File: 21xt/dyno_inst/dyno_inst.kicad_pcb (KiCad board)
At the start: 4 copper layers, 160 parts, among them IC1 MCP1502T-25E_CHY, IC2 TC7660SEOA713, IC3 MCP1502T-25E_CHY, J1 Conn_01x05, J3 Conn_01x03, J4 Barrel_Jack, J5 Conn_01x06, J6 Conn_01x04, U1 MAX14931FASE+, U10 LT3032IDE-5-TRPBF, U11 NCV8184DR2G, U12 1SS362FV_L3F, U13 1SS362FV_L3F, U14 ADA4807-2ARM, U15 ADA4807-2ARM, U16 ADA4945-1ACPZ-R2, U17 1SS362FV_L3F, U18 1SS362FV_L3F, U19 ADA4807-1, U2 MAX14930FASE+, U20 ADA4807-1, U22 ADA4945-1ACPZ-R2, U23 CPC1017N, U24 LT3032IDE-5-TRPBF, U3 AD7175-2BRUZ, U4 DEV-16771, U5 LT3032IDE-5-TRPBF, U6 1S4E_1.5U, U7 R-78E5.0-0.5, U8 TL431DBZ, U9 TL431DBZ

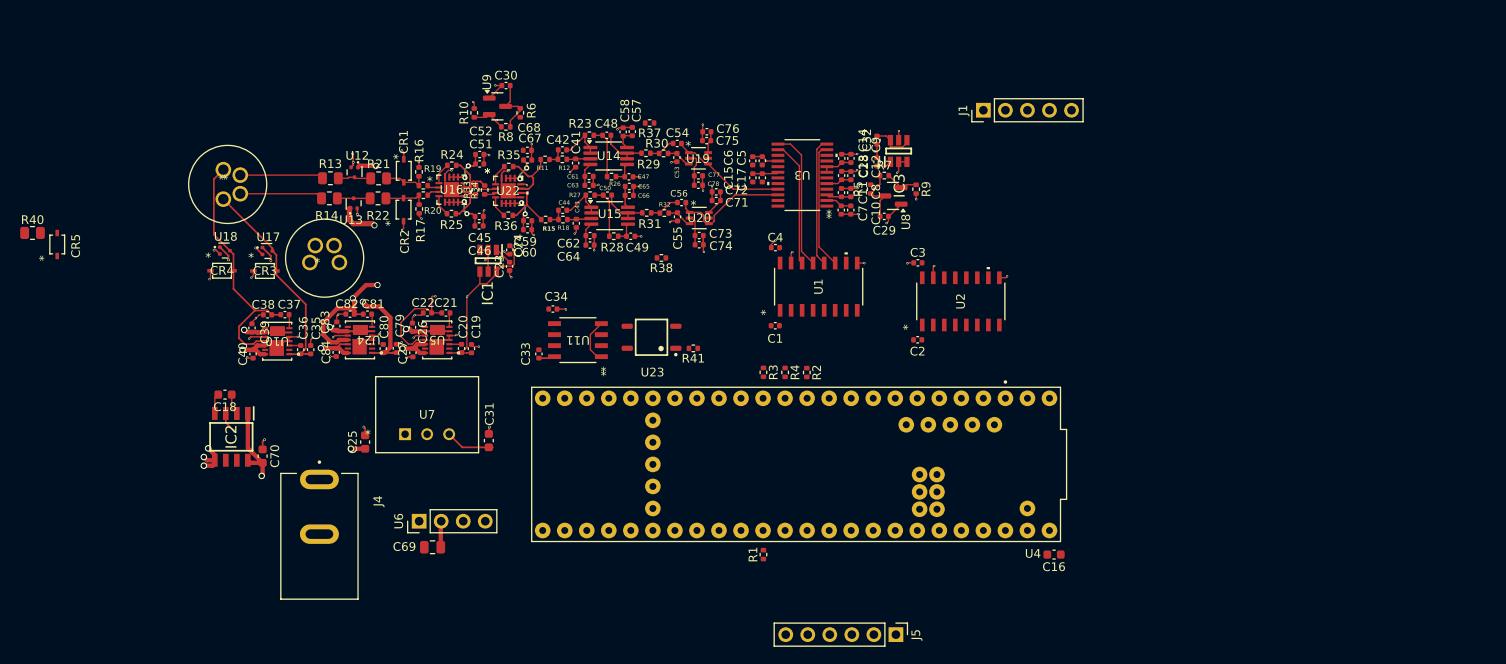
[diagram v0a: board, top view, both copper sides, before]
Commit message: scuffedd
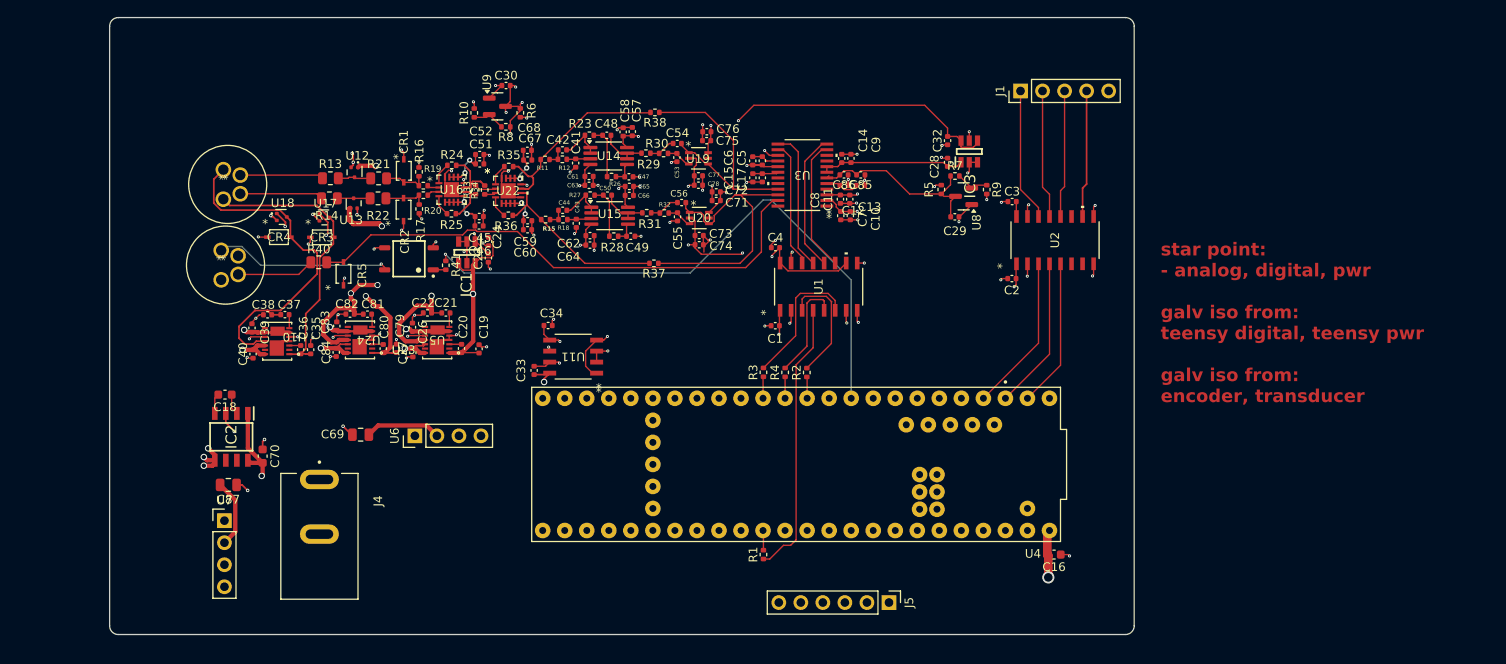
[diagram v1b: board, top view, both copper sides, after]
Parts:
- removed C25, C31: 10uF, Capacitor_SMD:C_0603_1608Metric
- added C85: 1uF, Capacitor_SMD:C_0402_1005Metric, F.Cu at (190.7, 71.5)
- added C86: 0.1uF, Capacitor_SMD:C_0402_1005Metric, F.Cu at (188.8, 71.5)
- added C87: 100uF, Capacitor_SMD:C_0805_2012Metric, F.Cu at (117.8, 107.2)
- U7: value R-78E5.0-0.5 -> 1S4E_1.5U; footprint dynoinst_fp:R-78E-0.5_RCP -> Connector_PinHeader_2.54mm:PinHeader_1x04_P2.54mm_Vertical
- moved CR5 33.2 mm to (131.1, 82.9)
- moved R40 33.2 mm to (128.2, 81.5)
- moved R41 30.1 mm to (142.9, 81.9), turned to -90 degrees
- moved U23 29.4 mm to (138.7, 81.2)
- moved U7 23.1 mm to (117.4, 111.3)
- moved R38 16.8 mm to (167.0, 64.3)
- moved R37 16.2 mm to (166.9, 81.7)
- moved C69 15.4 mm to (133.1, 101.4)
- moved C2 13.0 mm to (208.2, 83.4)
- moved C3 13.0 mm to (208.2, 74.6)
- moved U2 13.0 mm to (213.1, 79.0)
- moved J3 11.5 mm to (117.5, 81.9), turned to -90 degrees
- moved U6 9.86 mm to (139.3, 101.6)
- moved C28 8.14 mm to (200.7, 70.0)
- moved C32 8.14 mm to (200.7, 67.5)
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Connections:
- C1 pad 1: GND3 -> GNDA
- C15 pad 1: GNDD -> GNDA
- C17 pad 1: GNDD -> GNDA
- C2 pad 1: GND2 -> GNDA
- C3 pad 1: GNDD -> GND2
- C33 pad 1: GND2 -> GNDA
- C33 pad 2: 5venc -> 5vpwr
- C34 pad 1: GNDD -> GNDA
- C4 pad 1: GNDD -> GNDA
- C5 pad 2: GNDD -> GNDA
- C6 pad 2: GNDD -> GNDA
- J3 pad 1: ACSIG -> GND1
- J3 pad 2: GND1 -> ACSIG
- U1 pad 15: GNDD -> GNDA
- U1 pad 2: GND2 -> GNDA
- U1 pad 8: GND2 -> GNDA
- U1 pad 9: GNDD -> GNDA
- U11 pad 2: GND2 -> GNDA
- U11 pad 3: GND2 -> GNDA
- U11 pad 6: GND2 -> GNDA
- U11 pad 7: GND2 -> GNDA
- U11 pad 8: 5venc -> 5vpwr
- U2 pad 15: GNDD -> GND2
- U2 pad 2: GND2 -> GNDA
- U2 pad 8: GND2 -> GNDA
- U2 pad 9: GNDD -> GND2
- U23 pad 2: GND3 -> GNDA
- U3 pad 15: GNDD -> GNDA
- U3 pad 17: GNDD -> GNDA
- U4 pad 0: Benc1 -> Benc3
- U4 pad 2: unconnected-(U4-OUT2-Pad2) -> Benc1
- U4 pad 7: Benc3 -> unconnected-(U4-RX2-Pad7)
- U7 pad 1: +12v -> GNDPWR
- U7 pad 2: GNDPWR -> +12v
- U7 pad 3: 5venc -> GND2
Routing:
- net 5venc: track 7.54 -> 195.7 mm
- net 5vpwr: track 0.00 -> 102.2 mm, vias 0 -> 2
- net shcalctrl: track 0.00 -> 69.4 mm, vias 0 -> 1
- net ACSIG^: track 0.00 -> 61.3 mm
- net -5vref: track 25.8 -> 80.2 mm, vias 1 -> 8
- net +5vref: track 36.9 -> 84.3 mm, vias 1 -> 6
- net 3v3Ext: track 5.14 -> 44.2 mm, vias 0 -> 2
- net GNDA: track 83.8 -> 117.7 mm, vias 51 -> 70
- net ASCLK: track 0.00 -> 32.0 mm
- net ACSHCAL: track 0.00 -> 20.4 mm, vias 0 -> 1
- net +DCSIG^'*: track 14.5 -> 33.6 mm
- net Benc1: track 0.00 -> 18.1 mm
- net Benc2: track 0.00 -> 17.6 mm
- net Benc3: track 0.00 -> 17.1 mm
- net AMISO: track 0.00 -> 15.8 mm
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- added copper zone on In2.Cu, net +5vref
- added copper zone on In2.Cu, net -5vref
- added copper zone on In2.Cu, net 3v3Teensy
- added copper zone on In1.Cu, net GND2
- added copper zone on In1.Cu, net GND3
- removed copper zone on In1.Cu, net GNDD
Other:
- board outline added: 118.1 x 71.1 mm
- board text added: "star point: - analog, digital, pwr galv iso from: teensy digital, teensy pwr galv iso from: encoder, transducer"
